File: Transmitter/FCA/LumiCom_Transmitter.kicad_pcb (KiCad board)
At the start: 4 copper layers, 50 x 42 mm, 38 parts, among them J1 V, J2 IN_B, J3 IN_A, J4 OUT_B, J5 OUT_A, U1 OPA2675

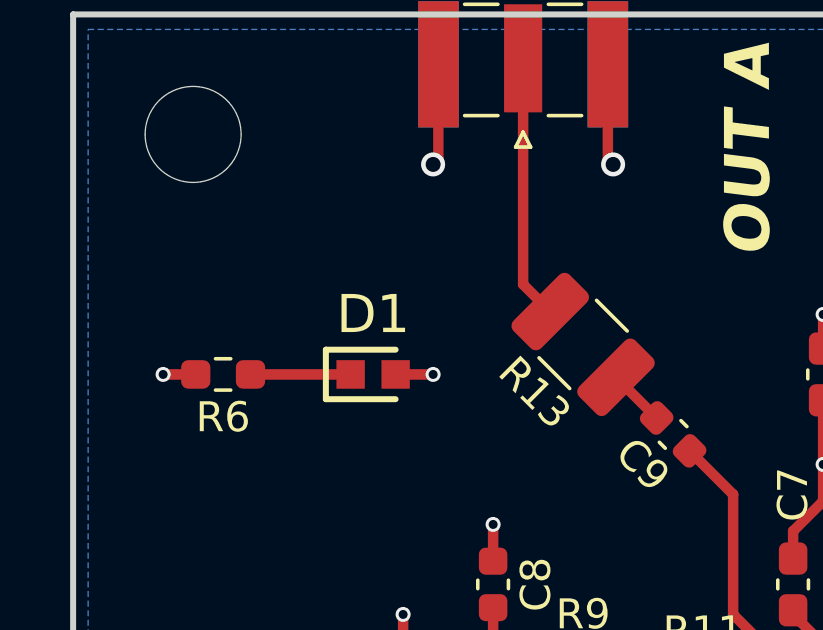
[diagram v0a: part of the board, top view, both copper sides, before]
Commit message: Small updates
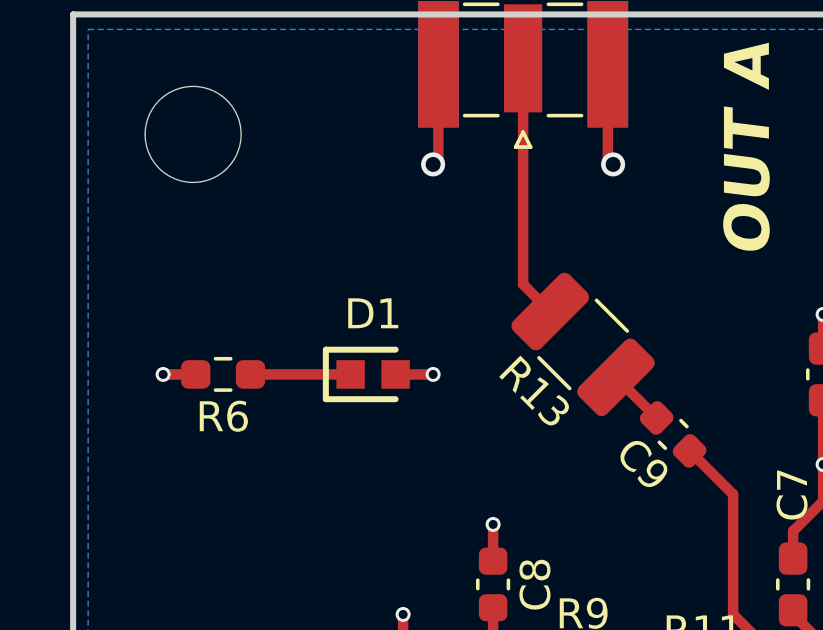
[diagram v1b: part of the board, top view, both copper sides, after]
